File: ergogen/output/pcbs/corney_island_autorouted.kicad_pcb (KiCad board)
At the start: 2 copper layers, 133.8 x 91.7 mm, 94 parts

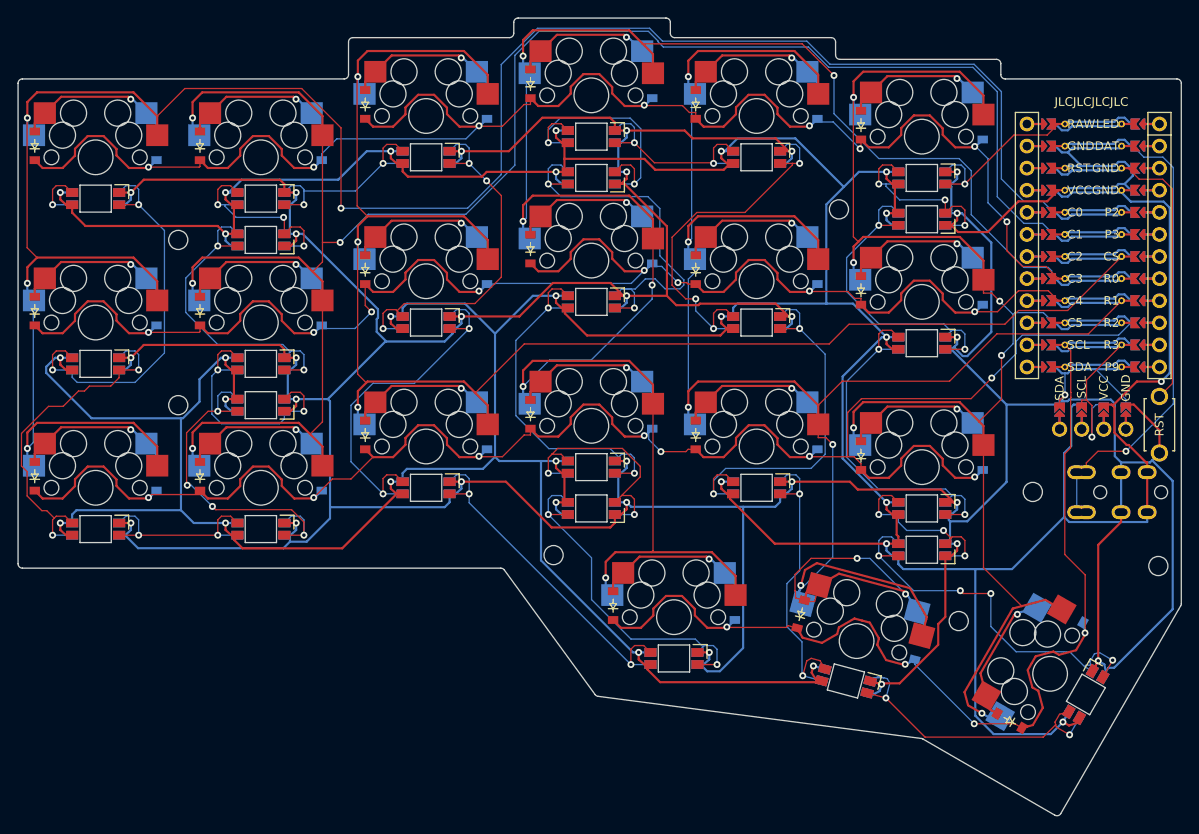
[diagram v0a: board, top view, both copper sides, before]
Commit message: Update assets
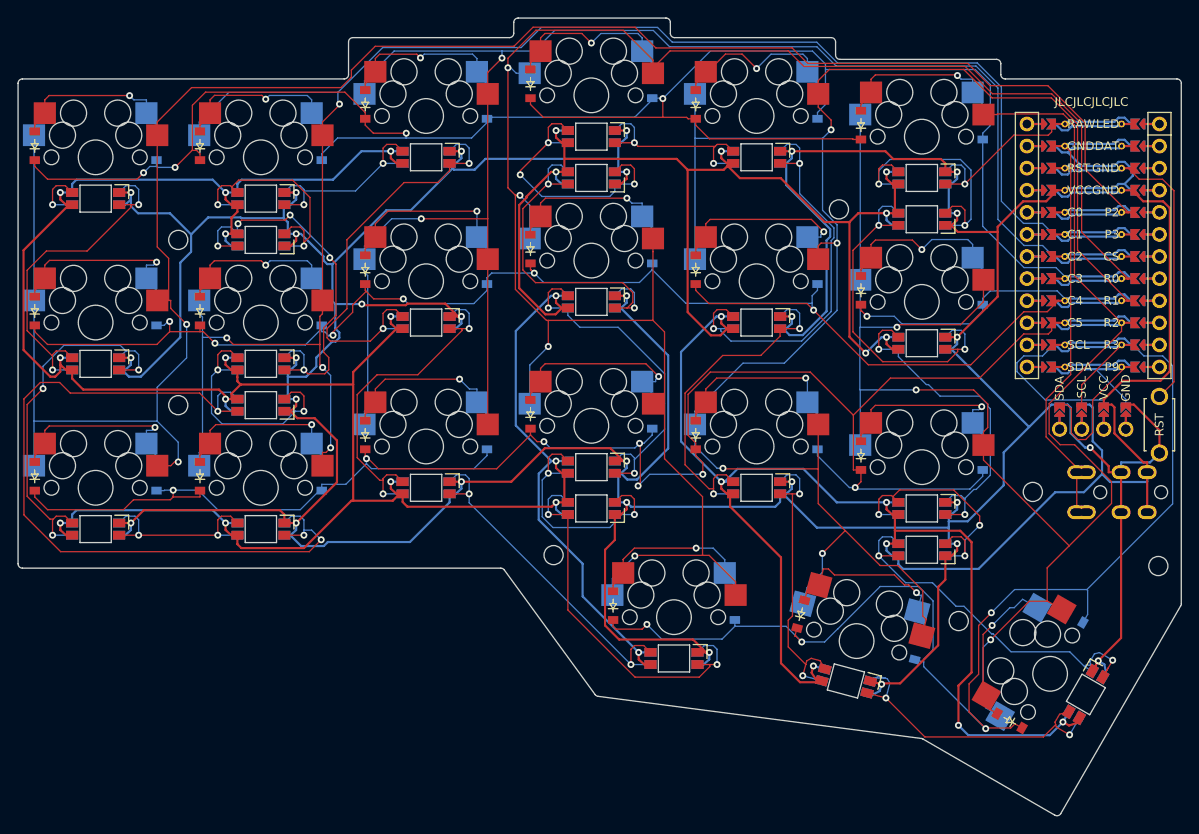
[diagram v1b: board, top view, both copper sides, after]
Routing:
- net LED_17: track 40.9 -> 90.3 mm, vias 4 -> 3
- net R0: track 192.2 -> 230.1 mm, vias 8 -> 4
- net C5: track 165.7 -> 201.0 mm, vias 6 -> 3
- net VCC: track 644.6 -> 678.9 mm, vias 28 -> 29
- net C0: track 258.8 -> 237.8 mm, vias 4 -> 2
- net R3: track 127.0 -> 146.5 mm
- net C1: track 229.2 -> 210.2 mm
- net mid_home: track 40.6 -> 21.8 mm, vias 2 -> 1
- net R2: track 202.0 -> 220.4 mm, vias 8 -> 7
- net R1: track 182.4 -> 198.9 mm, vias 8 -> 7
- net GND: track 636.6 -> 622.9 mm, vias 27 -> 29
- net SDA: track 19.6 -> 32.2 mm, vias 1 -> 0
- net C4: track 200.8 -> 212.9 mm, vias 5 -> 4
- net LED_1: track 22.8 -> 33.4 mm, vias 3 -> 2
- net ULED_2: track 21.2 -> 30.4 mm
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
